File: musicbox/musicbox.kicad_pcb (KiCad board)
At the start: 2 copper layers, 41 x 62.5 mm, 21 parts, among them J1 USB_C_Receptacle_USB2.0_14P, J10 JBL_CONNECTOR, J2 JST_PH_2pin, J3 PN532_SPI, J4 PCM5102A_I2S, J7 BUTTONS_CONN, J8 ESP_LEFT, J9 ESP_RIGHT, Q1 BC547, Q2 BC547, Q3 BC547

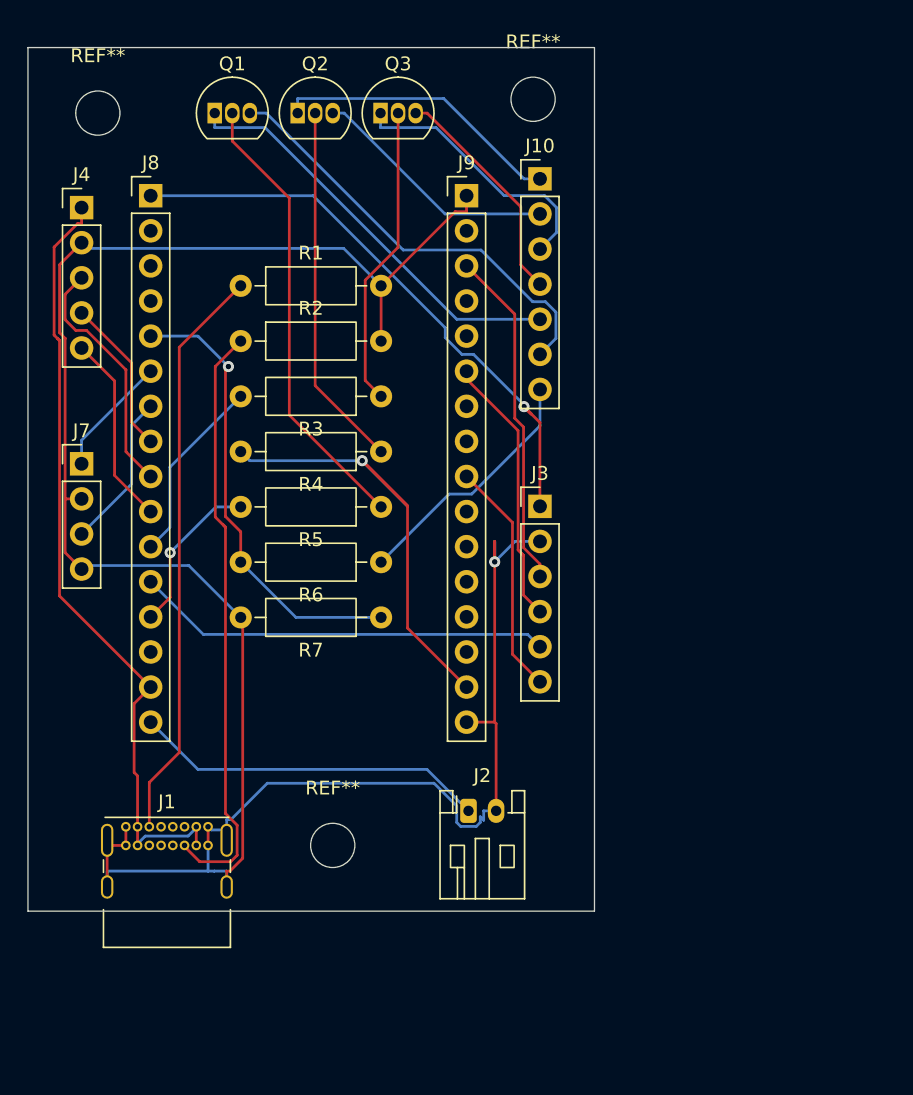
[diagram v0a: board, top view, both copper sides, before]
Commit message: mvp
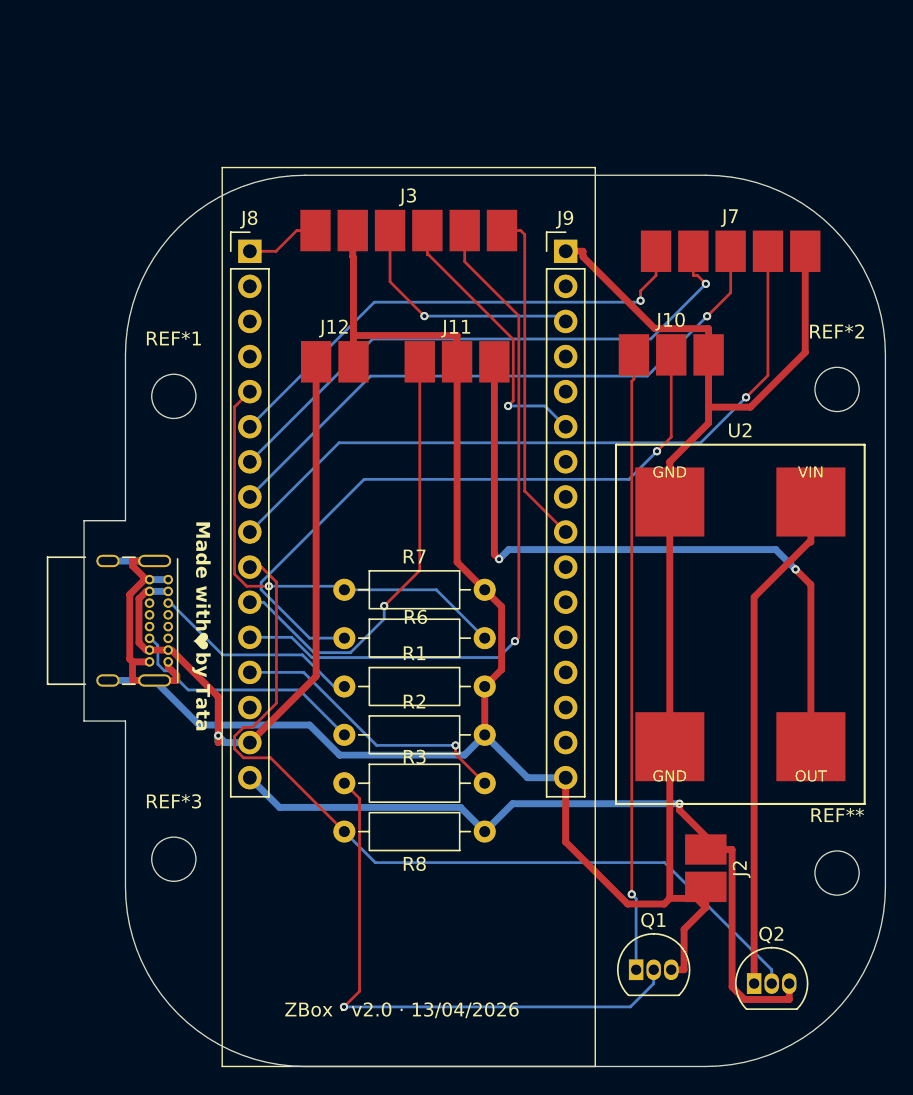
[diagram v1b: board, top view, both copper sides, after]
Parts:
- removed J4: PCM5102A_I2S, Connector_PinHeader_2.54mm:PinHeader_1x05_P2.54mm_Vertical
- removed Q3: BC547, Package_TO_SOT_THT:TO-92_Inline
- removed R4, R5: 2.2k, Resistor_THT:R_Axial_DIN0207_L6.3mm_D2.5mm_P10.16mm_Horizontal
- removed the REF** at (88.0, 53.0)
- removed the REF** at (105.0, 106.0)
- removed the REF** at (119.5, 52.0)
- added G***: LOGO, musicbox_o:Untitled, F.Cu at (95.5, 91.2)
- added J11: PAD_LED_WS2812B, musicbox:SolderPad_1x03_W2.2mm_H3mm_P2.7mm, F.Cu at (114.0, 71.0)
- added J12: PAD_JBL_PWR, musicbox:SolderPad_1x02_W2.2mm_H3mm_P2.7mm, F.Cu at (105.2, 71.0)
- added R8: 100k, Resistor_THT:R_Axial_DIN0207_L6.3mm_D2.5mm_P10.16mm_Horizontal, F.Cu at (116.0, 105.0)
- added REF**: MountingHole_3.2mm_M3, MountingHole:MountingHole_3.2mm_M3, F.Cu at (141.5, 108.0)
- added REF*1: MountingHole_3.2mm_M3, MountingHole:MountingHole_3.2mm_M3, F.Cu at (93.5, 73.5)
- added REF*2: MountingHole_3.2mm_M3, MountingHole:MountingHole_3.2mm_M3, F.Cu at (141.5, 73.0)
- added REF*3: MountingHole_3.2mm_M3, MountingHole:MountingHole_3.2mm_M3, F.Cu at (93.5, 107.0)
- added U2: STEPUP_MT3608, musicbox:MT3608_Pancake, F.Cu at (134.5, 90.0)
- J10: value JBL_CONNECTOR -> PAD_JBL; footprint Connector_PinHeader_2.54mm:PinHeader_1x07_P2.54mm_Vertical -> musicbox:SolderPad_1x03_W2.2mm_H3mm_P2.7mm
- J2: value JST_PH_2pin -> PAD_BAT_LIPO; footprint Connector_JST:JST_PH_S2B-PH-K_1x02_P2.00mm_Horizontal -> musicbox:SolderPad_1x02_W2.2mm_H3mm_P2.7mm
- J3: value PN532_SPI -> PAD_PN532_SPI; footprint Connector_PinHeader_2.54mm:PinHeader_1x06_P2.54mm_Vertical -> musicbox:SolderPad_1x06_W2.2mm_H3mm_P2.7mm
- J7: value BUTTONS_CONN -> PAD_BUTTONS; footprint Connector_PinHeader_2.54mm:PinHeader_1x04_P2.54mm_Vertical -> musicbox:SolderPad_1x05_W2.2mm_H3mm_P2.7mm
- Q2: value BC547 -> BS250
- moved Q2 71.1 mm to (135.5, 116.0)
- moved Q1 69.1 mm to (127.0, 115.0)
- moved J7 49.4 mm to (133.8, 63.0)
- moved R1 30.0 mm to (105.8, 94.5)
- moved R2 29.5 mm to (105.8, 98.0)
- moved R3 28.1 mm to (105.8, 101.5), turned to 0 degrees
- moved J3 22.1 mm to (110.5, 61.5)
- moved J1 18.1 mm to (93.1, 86.8), turned to -90 degrees
- moved J2 17.7 mm to (132.0, 107.7), turned to -90 degrees
- moved J10 15.9 mm to (129.5, 70.5)
- moved J8 8.22 mm to (99.0, 63.0)
- moved J9 8.22 mm to (121.9, 63.0)
- moved R6 6.11 mm to (105.8, 91.0), turned to 0 degrees
- moved R7 3.33 mm to (105.8, 87.5), turned to 0 degrees
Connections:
- J10 pad 1: Net-(J10-Pin_1) -> /JBL_BTN_P
- J10 pad 2: Net-(J10-Pin_2) -> /JBL_LINE
- J10 pad 3: Net-(J10-Pin_3) -> GND
- J2 pad 1: Net-(J2-Pin_1) -> /BAT
- J7 pad 2: GND -> /BTN_B (VOL-)
- J7 pad 3: /BTN_B (VOL-) -> /BTN_C
- J7 pad 4: GND -> /BTN_D
- J8 pad 10: /I2S_DIN -> /LED_EN
- J8 pad 11: /JBL_VOL+ -> /LED_DIN
- J8 pad 16: Net-(J2-Pin_1) -> /BAT
- J8 pad 8: /I2S_LRCK -> /BTN_C
- J8 pad 9: /I2S_BCK -> /BTN_D
- J9 pad 15: /JBL_VOL- -> unconnected-(J9-Pin_15-Pad15)
- Q1 pad 1: Net-(J10-Pin_5) -> /JBL_BTN_P
- Q1 pad 3: Net-(J10-Pin_6) -> GND
- Q2 pad 1: Net-(J10-Pin_1) -> Net-(Q2-D)
- Q2 pad 2: Net-(Q2-B) -> /LED_EN
- Q2 pad 3: Net-(J10-Pin_2) -> /BAT
- R3 pad 1: Net-(Q3-B) -> Net-(Q1-B)
- R3 pad 2: /JBL_VOL+ -> /JBL_PWR
- R6 pad 1: Net-(J10-Pin_7) -> /JBL_LINE
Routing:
- net /LED_EN: track 0.00 -> 62.6 mm
- net /BAT: track 0.00 -> 55.6 mm, vias 0 -> 1
- net /BTN_D: track 0.00 -> 51.2 mm, vias 0 -> 1
- net /+5V_LED: track 0.00 -> 50.0 mm, vias 0 -> 2
- net /JBL_LINE: track 0.00 -> 48.0 mm, vias 0 -> 1
- net /JBL_VOL-: track 47.1 -> 0.00 mm, vias 1 -> 0
- net /JBL_BTN_P: track 0.00 -> 44.7 mm, vias 0 -> 1
- net /BTN_C: track 0.00 -> 43.9 mm, vias 0 -> 1
- net +3V3: track 44.7 -> 5.37 mm, vias 1 -> 0
- net Net-(Q2-D): track 0.00 -> 36.6 mm
- net /LED_DIN: track 0.00 -> 31.9 mm, vias 0 -> 1
- net Net-(J10-Pin_6): track 31.6 -> 0.00 mm
- net Net-(J10-Pin_5): track 30.3 -> 0.00 mm
- net GND: track 173.0 -> 203.2 mm, vias 1 -> 0
- net /BTN_B (VOL-): track 11.3 -> 41.2 mm, vias 0 -> 1
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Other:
- board size 41 x 62.5 mm -> 58 x 64.5 mm
- board text added: "Made with by Tata"
- board text added: "ZBox · v2.0 · 13/04/2026"
